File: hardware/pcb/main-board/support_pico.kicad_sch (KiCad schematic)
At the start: 27 parts, among them J701 Conn_01x02, J702 Z88 SD Card, U702 RP2040, U703 W25Q128JVS, Y701 ABLS-12.000MHZ-B4-T

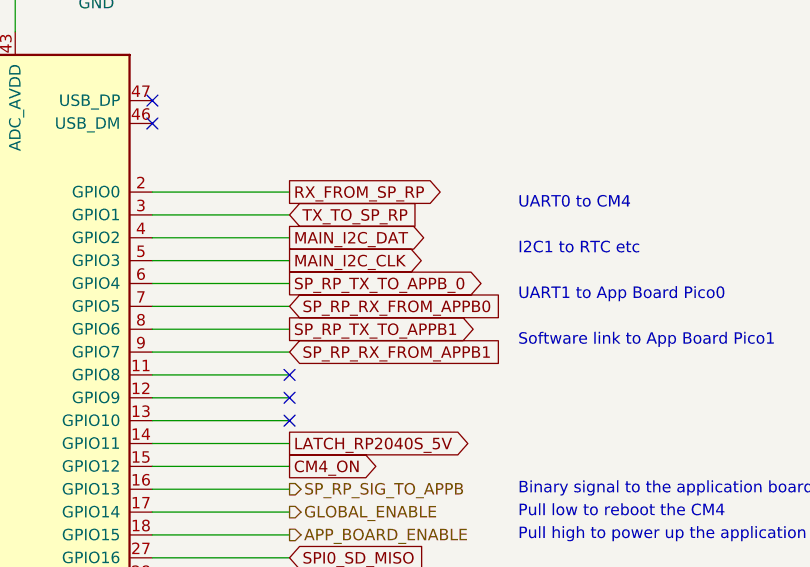
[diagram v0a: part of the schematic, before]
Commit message: tidy the keyboard comms
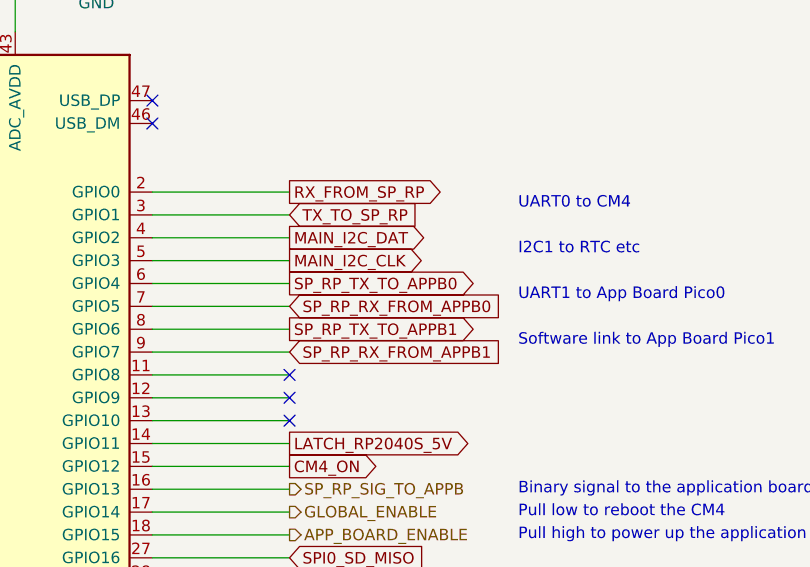
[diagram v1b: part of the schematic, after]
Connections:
- net SP_RP_TX_TO_APPB_0 renamed SP_RP_TX_TO_APPB0
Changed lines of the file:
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@@
 		)
 	)
-	(global_label "SP_RP_TX_TO_APPB_0"
+	(global_label "SP_RP_TX_TO_APPB0"
 		(shape output)
 		(at 113.03 81.28 0)
@@
 		)
 		(property "Intersheetrefs" "${INTERSHEET_REFS}"
-			(at 135.8018 81.28 0)
+			(at 134.8342 81.28 0)
 			(effects
 				(font
